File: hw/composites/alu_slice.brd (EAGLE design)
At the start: 50 x 50 mm, 13 parts, among them CON2 GENERIC-2X10

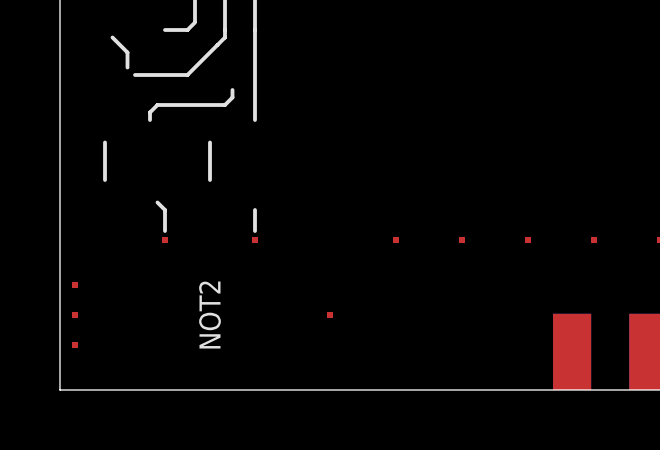
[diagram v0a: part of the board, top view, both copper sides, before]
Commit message: Basic cleanups
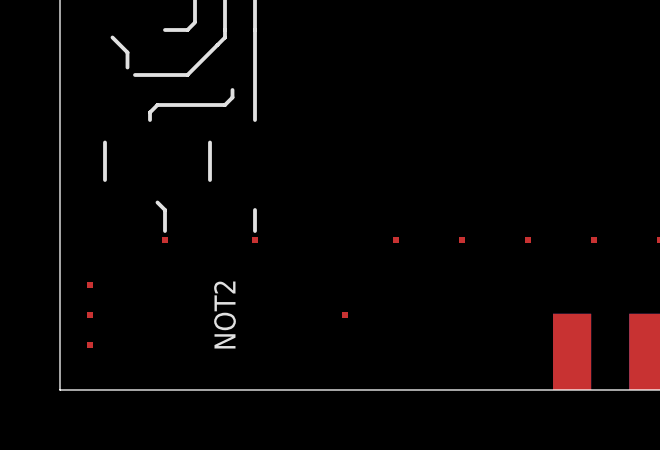
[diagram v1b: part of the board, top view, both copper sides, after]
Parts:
- moved NOT2 0.50 mm to (9.50, 0.50)
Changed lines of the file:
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@@
 <setting verticaltext="up"/>
 </settings>
-<grid distance="0.1" unitdist="mm" unit="mm" style="lines" multiple="1" display="yes" altdistance="0.02" altunitdist="mm" altunit="mm"/>
+<grid distance="0.5" unitdist="mm" unit="mm" style="lines" multiple="1" display="yes" altdistance="0.02" altunitdist="mm" altunit="mm"/>
 <layers>
 <layer number="1" name="Top" color="4" fill="1" visible="yes" active="yes"/>
@@
 <layer number="20" name="Dimension" color="15" fill="1" visible="yes" active="yes"/>
 <layer number="21" name="tPlace" color="7" fill="1" visible="yes" active="yes"/>
-<layer number="22" name="bPlace" color="7" fill="1" visible="yes" active="yes"/>
+<layer number="22" name="bPlace" color="7" fill="1" visible="no" active="yes"/>
 <layer number="23" name="tOrigins" color="15" fill="1" visible="yes" active="yes"/>
-<layer number="24" name="bOrigins" color="15" fill="1" visible="yes" active="yes"/>
+<layer number="24" name="bOrigins" color="15" fill="1" visible="no" active="yes"/>
 <layer number="25" name="tNames" color="7" fill="1" visible="no" active="yes"/>
 <layer number="26" name="bNames" color="7" fill="1" visible="no" active="yes"/>
@@
 <layer number="38" name="bTest" color="7" fill="1" visible="no" active="yes"/>
 <layer number="39" name="tKeepout" color="4" fill="11" visible="yes" active="yes"/>
-<layer number="40" name="bKeepout" color="1" fill="11" visible="yes" active="yes"/>
+<layer number="40" name="bKeepout" color="1" fill="11" visible="no" active="yes"/>
 <layer number="41" name="tRestrict" color="4" fill="10" visible="yes" active="yes"/>
-<layer number="42" name="bRestrict" color="1" fill="10" visible="yes" active="yes"/>
+<layer number="42" name="bRestrict" color="1" fill="10" visible="no" active="yes"/>
 <layer number="43" name="vRestrict" color="2" fill="10" visible="no" active="yes"/>
 <layer number="44" name="Drills" color="7" fill="1" visible="no" active="yes"/>
@@
 <layer number="49" name="Reference" color="7" fill="1" visible="no" active="yes"/>
 <layer number="50" name="dxf" color="7" fill="1" visible="no" active="no"/>
-<layer number="51" name="tDocu" color="7" fill="1" visible="no" active="yes"/>
+<layer number="51" name="tDocu" color="7" fill="1" visible="yes" active="yes"/>
 <layer number="52" name="bDocu" color="7" fill="1" visible="no" active="yes"/>
 <layer number="53" name="tGND_GNDA" color="7" fill="9" visible="no" active="no"/>
@@
 <autorouter>
 <pass name="Default">
-<param name="RoutingGrid" value="50mil"/>
-<param name="AutoGrid" value="1"/>
-<param name="Efforts" value="0"/>
-<param name="TopRouterVariant" value="1"/>
+<param name="RoutingGrid" value="0.05mm"/>
+<param name="AutoGrid" value="0"/>
+<param name="Efforts" value="2"/>
+<param name="TopRouterVariant" value="0"/>
 <param name="tpViaShape" value="round"/>
-<param name="PrefDir.1" value="|"/>
+<param name="PrefDir.1" value="-"/>
 <param name="PrefDir.2" value="0"/>
 <param name="PrefDir.3" value="0"/>
@@
 <param name="PrefDir.14" value="0"/>
 <param name="PrefDir.15" value="0"/>
-<param name="PrefDir.16" value="-"/>
+<param name="PrefDir.16" value="|"/>
 <param name="cfVia" value="8"/>
 <param name="cfNonPref" value="5"/>
@@
 <element name="SEL1" library="p.peter-gator" package="SELECTOR-2-LANE-NOMUX" value="1_BIT_SELECT" x="0.5" y="34.5"/>
 <element name="SEL3" library="p.peter-gator" package="SELECTOR-2-LANE-NOMUX" value="1_BIT_SELECT" x="12.5" y="34.5"/>
-<element name="NOT2" library="p.peter-gator" package="NOT-VERTICAL" value="NOTVERTICAL" x="9" y="0.5" rot="R90"/>
+<element name="NOT2" library="p.peter-gator" package="NOT-VERTICAL" value="NOTVERTICAL" x="9.5" y="0.5" rot="R90"/>
 <element name="NAND1" library="p.peter-gator" package="NAND" value="NAND" x="0.5" y="5"/>
 <element name="XOR4" library="p.peter-gator" package="XOR" value="XOR" x="28.5" y="19.5"/>
@@
 <wire x1="1.5" y1="32" x2="11.5" y2="34.5" width="0" layer="19" extent="1-1"/>
 <wire x1="4.5" y1="13.5" x2="1.5" y2="32" width="0" layer="19" extent="1-1"/>
-<wire x1="0.5" y1="3.5" x2="4.5" y2="13.5" width="0" layer="19" extent="1-1"/>
+<wire x1="1" y1="3.5" x2="4.5" y2="13.5" width="0" layer="19" extent="1-1"/>
 <wire x1="48" y1="5" x2="48.5" y2="32" width="0" layer="19" extent="1-1"/>
 <wire x1="39.93" y1="1.27" x2="48" y2="5" width="0" layer="19" extent="1-16"/>
@@
 <wire x1="9.5" y1="34.5" x2="13.8" y2="32" width="0" layer="19" extent="1-1"/>
 <wire x1="6.5" y1="13.5" x2="13.8" y2="32" width="0" layer="19" extent="1-1"/>
-<wire x1="0.5" y1="2.5" x2="6.5" y2="13.5" width="0" layer="19" extent="1-1"/>
+<wire x1="1" y1="2.5" x2="6.5" y2="13.5" width="0" layer="19" extent="1-1"/>
 <wire x1="46" y1="5" x2="47.5" y2="32" width="0" layer="19" extent="1-1"/>
 <wire x1="39.93" y1="1.27" x2="46" y2="5" width="0" layer="19" extent="1-1"/>
@@
 <contactref element="SEL1" pad="SEL"/>
 <contactref element="NOT2" pad="A"/>
-<wire x1="9" y1="2.5" x2="2.5" y2="34.5" width="0" layer="19" extent="1-1"/>
+<wire x1="9.5" y1="2.5" x2="2.5" y2="34.5" width="0" layer="19" extent="1-1"/>
 </signal>
 <signal name="INV_ADD">
@@
 <contactref element="NAND1" pad="A"/>
 <contactref element="NOT2" pad="NOT"/>
-<wire x1="0.5" y1="1.5" x2="3.5" y2="5" width="0" layer="19" extent="1-1"/>
+<wire x1="1" y1="1.5" x2="3.5" y2="5" width="0" layer="19" extent="1-1"/>
 </signal>
 <signal name="N$3">
